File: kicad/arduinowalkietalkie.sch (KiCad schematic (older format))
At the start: 32 parts, among them SW1 SW_Push_Dual, SW10 SW_Push_Dual, SW11 SW_Push_Dual, SW12 SW_Push_Dual, SW13 SW_Push_Dual, SW14 SW_Push_Dual, SW2 SW_Push_Dual, SW3 SW_Push_Dual, SW4 SW_Push_Dual, SW5 SW_Push_Dual, SW6 SW_Push_Dual, SW7 SW_Push_Dual, SW8 SW_Push_Dual, SW9 SW_Push_Dual, U1 NRF24L01_Breakout

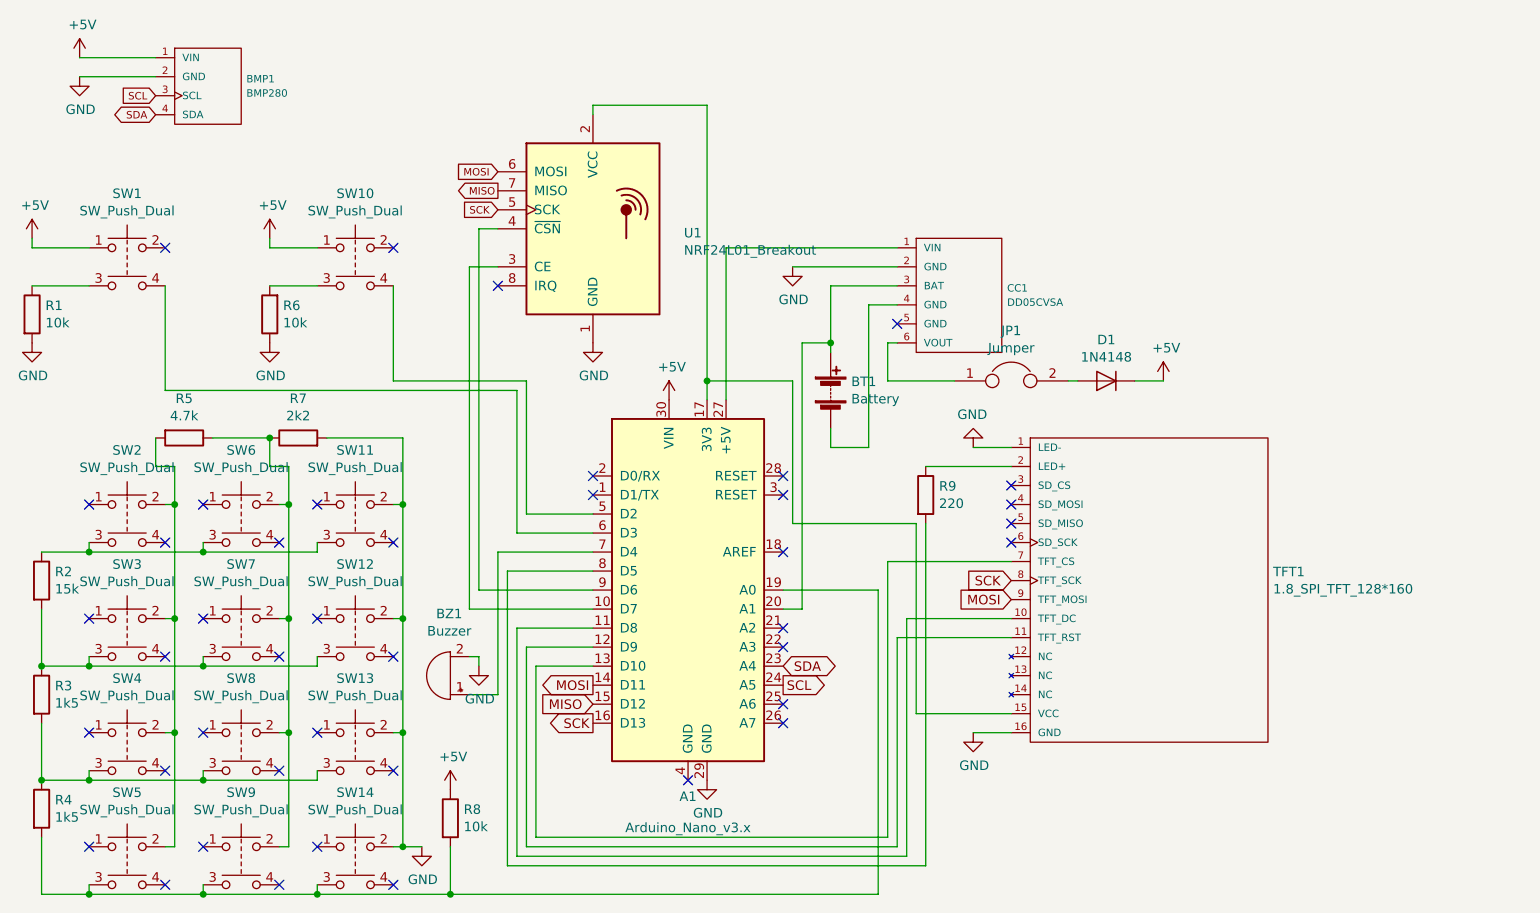
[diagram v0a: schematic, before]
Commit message: update pcb
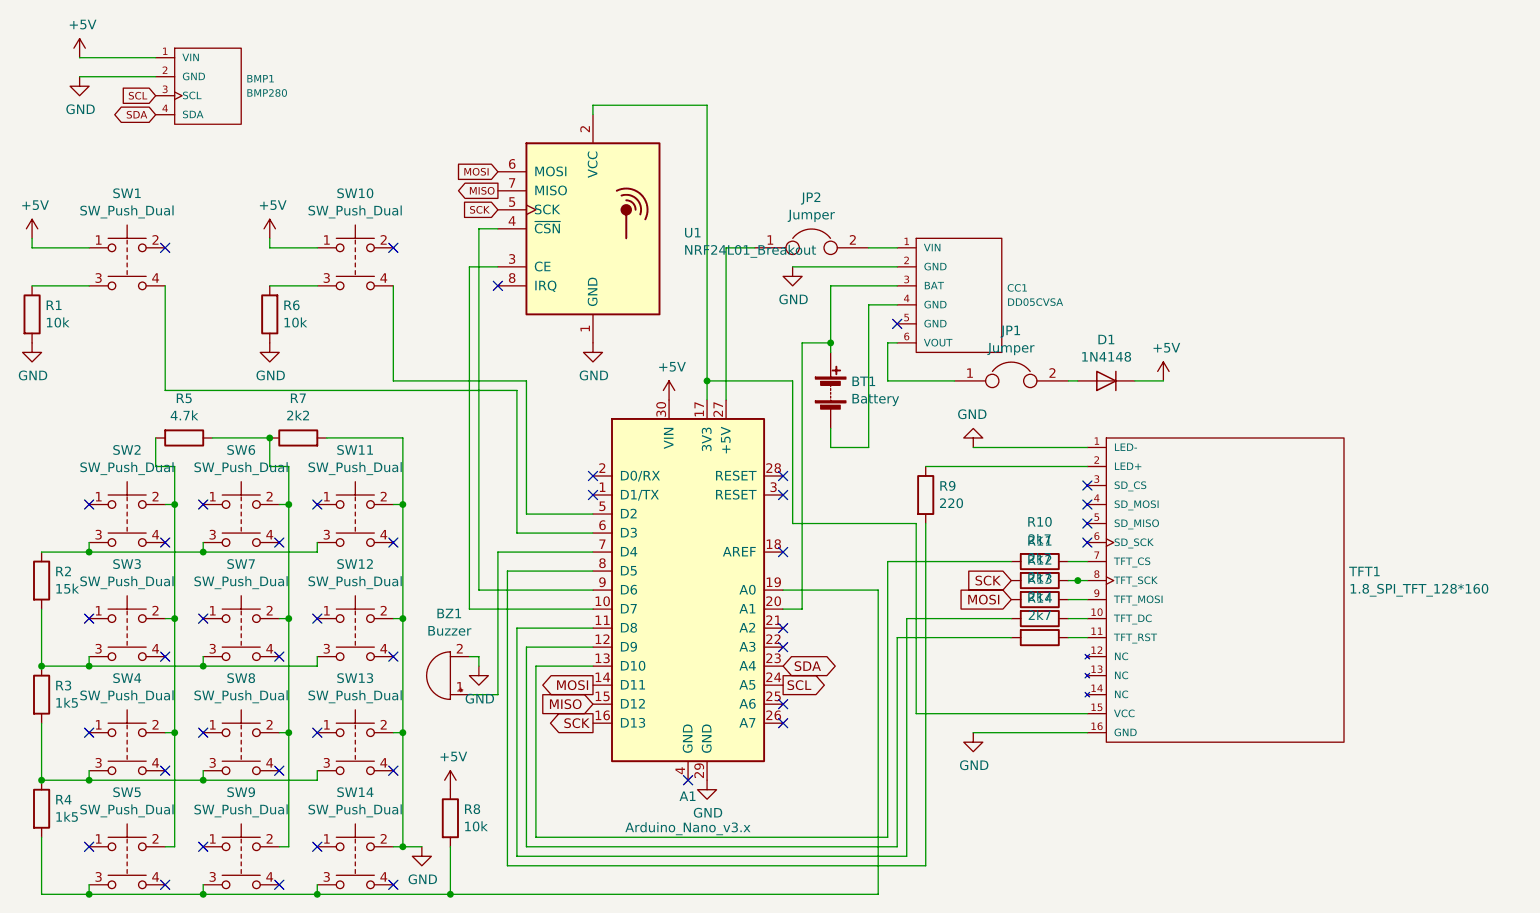
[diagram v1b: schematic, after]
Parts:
- added JP2: Jumper, PIN_JUMPER:PIN_JUMPER, symbol Device:Jumper
- added R10, R11, R12, R13, R14: 2k7, Resistor_THT:R_Axial_DIN0207_L6.3mm_D2.5mm_P7.62mm_Horizontal, symbol Device:R
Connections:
- net MOSI: now also R12.2; no longer TFT1.9 (TFT_MOSI)
- net SCK: now also R11.2; no longer TFT1.8 (TFT_SCK)
- net at A1.11 (D8): now also R13.2; no longer TFT1.10 (TFT_DC)
- net at A1.12 (D9): now also R14.2; no longer TFT1.11 (TFT_RST)
- net at A1.13 (D10): now also R10.2; no longer TFT1.7 (TFT_CS)
- net at A1.27 (+5V): now also JP2.1; no longer CC1.1 (VIN)
- new net: R13.1, TFT1.10 (TFT_DC)
- new net: R14.1, TFT1.11 (TFT_RST)
- new net: R10.1, TFT1.7 (TFT_CS)
- new net: R11.1, TFT1.8 (TFT_SCK)
- new net: R12.1, TFT1.9 (TFT_MOSI)
- new net: CC1.1 (VIN), JP2.2
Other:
- moved on the sheet: TFT1
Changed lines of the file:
@@
 L TFT_KMR-1.8_SPI:1.8_SPI_TFT_128*160 TFT1
 U 1 1 5C5E391F
-P 7300 3850
-F 0 "TFT1" H 8777 3146 50  0000 L CNN
-F 1 "1.8_SPI_TFT_128*160" H 8777 3055 50  0000 L CNN
-F 2 "TFT_KMR_18_SPI:TFT_KMR_1.8_SPI" H 7300 3850 50  0001 C CNN
-F 3 "" H 7300 3850 50  0001 C CNN
-	1    7300 3850
+P 7700 3850
+F 0 "TFT1" H 9177 3146 50  0000 L CNN
+F 1 "1.8_SPI_TFT_128*160" H 9177 3055 50  0000 L CNN
+F 2 "TFT_KMR_18_SPI:TFT_KMR_1.8_SPI" H 7700 3850 50  0001 C CNN
+F 3 "" H 7700 3850 50  0001 C CNN
+	1    7700 3850
 	1    0    0    -1
 $EndComp
@@
 	1    0    0    -1
 $EndComp
-Wire Wire Line
-	7200 5400 7400 5400
 Text GLabel 5200 5150 0    50   Output ~ 0
 MOSI
@@
 	-1   0    0    1
 $EndComp
-Wire Wire Line
-	7200 3900 7400 3900
 Text GLabel 7400 4700 0    50   Input ~ 0
 MOSI
@@
 	5900 3650 5900 2850
 Wire Wire Line
-	5900 2850 6800 2850
+	5900 2850 6050 2850
 $Comp
 L power:GND #PWR012
@@
 $EndComp
 NoConn ~ 4700 3050
-NoConn ~ 7400 4100
-NoConn ~ 7400 4200
-NoConn ~ 7400 4300
-NoConn ~ 7400 4400
+NoConn ~ 7800 4100
+NoConn ~ 7800 4200
+NoConn ~ 7800 4300
+NoConn ~ 7800 4400
 NoConn ~ 2550 4200
 NoConn ~ 3150 4200
@@
 Wire Wire Line
 	6900 4300 6900 5300
-Wire Wire Line
-	6900 5300 7400 5300
 Connection ~ 5800 3550
 Wire Wire Line
 	5800 3550 5800 2100
-Wire Wire Line
-	7400 4000 6950 4000
 Wire Wire Line
 	6950 6100 4750 6100
@@
 Wire Wire Line
 	4600 5000 4600 5050
+$Comp
+L Device:R R10
+U 1 1 5C72199E
+P 7550 4500
+F 0 "R10" V 7343 4500 50  0000 C CNN
+F 1 "2k7" V 7434 4500 50  0000 C CNN
+F 2 "Resistor_THT:R_Axial_DIN0207_L6.3mm_D2.5mm_P7.62mm_Horizontal" V 7480 4500 50  0001 C CNN
+F 3 "~" H 7550 4500 50  0001 C CNN
+	1    7550 4500
+	0    1    1    0
+$EndComp
+Wire Wire Line
+	7700 4500 7800 4500
+Wire Wire Line
+	7700 4600 7750 4600
+Wire Wire Line
+	7700 4700 7800 4700
+Wire Wire Line
+	7800 4800 7700 4800
+Wire Wire Line
+	7700 4900 7800 4900
+Wire Wire Line
+	6900 5300 7800 5300
+Wire Wire Line
+	7200 5400 7800 5400
+Wire Wire Line
+	6950 4000 7800 4000
+Wire Wire Line
+	7200 3900 7800 3900
+$Comp
+L Device:R R11
+U 1 1 5C759F76
+P 7550 4600
+F 0 "R11" V 7343 4600 50  0000 C CNN
+F 1 "2k7" V 7434 4600 50  0000 C CNN
+F 2 "Resistor_THT:R_Axial_DIN0207_L6.3mm_D2.5mm_P7.62mm_Horizontal" V 7480 4600 50  0001 C CNN
+F 3 "~" H 7550 4600 50  0001 C CNN
+	1    7550 4600
+	0    1    1    0
+$EndComp
+Connection ~ 7750 4600
+Wire Wire Line
+	7750 4600 7800 4600
+$Comp
+L Device:R R12
+U 1 1 5C75A044
+P 7550 4700
+F 0 "R12" V 7343 4700 50  0000 C CNN
+F 1 "2k7" V 7434 4700 50  0000 C CNN
+F 2 "Resistor_THT:R_Axial_DIN0207_L6.3mm_D2.5mm_P7.62mm_Horizontal" V 7480 4700 50  0001 C CNN
+F 3 "~" H 7550 4700 50  0001 C CNN
+	1    7550 4700
+	0    1    1    0
+$EndComp
+$Comp
+L Device:R R13
+U 1 1 5C75A09A
+P 7550 4800
+F 0 "R13" V 7343 4800 50  0000 C CNN
+F 1 "2k7" V 7434 4800 50  0000 C CNN
+F 2 "Resistor_THT:R_Axial_DIN0207_L6.3mm_D2.5mm_P7.62mm_Horizontal" V 7480 4800 50  0001 C CNN
+F 3 "~" H 7550 4800 50  0001 C CNN
+	1    7550 4800
+	0    1    1    0
+$EndComp
+$Comp
+L Device:R R14
+U 1 1 5C75A0F2
+P 7550 4900
+F 0 "R14" V 7343 4900 50  0000 C CNN
+F 1 "2k7" V 7434 4900 50  0000 C CNN
+F 2 "Resistor_THT:R_Axial_DIN0207_L6.3mm_D2.5mm_P7.62mm_Horizontal" V 7480 4900 50  0001 C CNN
+F 3 "~" H 7550 4900 50  0001 C CNN
+	1    7550 4900
+	0    1    1    0
+$EndComp
+$Comp
+L Device:Jumper JP2
+U 1 1 5C75AD4F
+P 6350 2850
+F 0 "JP2" H 6350 3114 50  0000 C CNN
+F 1 "Jumper" H 6350 3023 50  0000 C CNN
+F 2 "PIN_JUMPER:PIN_JUMPER" H 6350 2850 50  0001 C CNN
+F 3 "~" H 6350 2850 50  0001 C CNN
+	1    6350 2850
+	1    0    0    -1
+$EndComp
+Wire Wire Line
+	6650 2850 6800 2850
 $EndSCHEMATC
